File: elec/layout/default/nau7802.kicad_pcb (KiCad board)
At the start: 2 copper layers, 225.7 x 100.8 mm, 0 parts

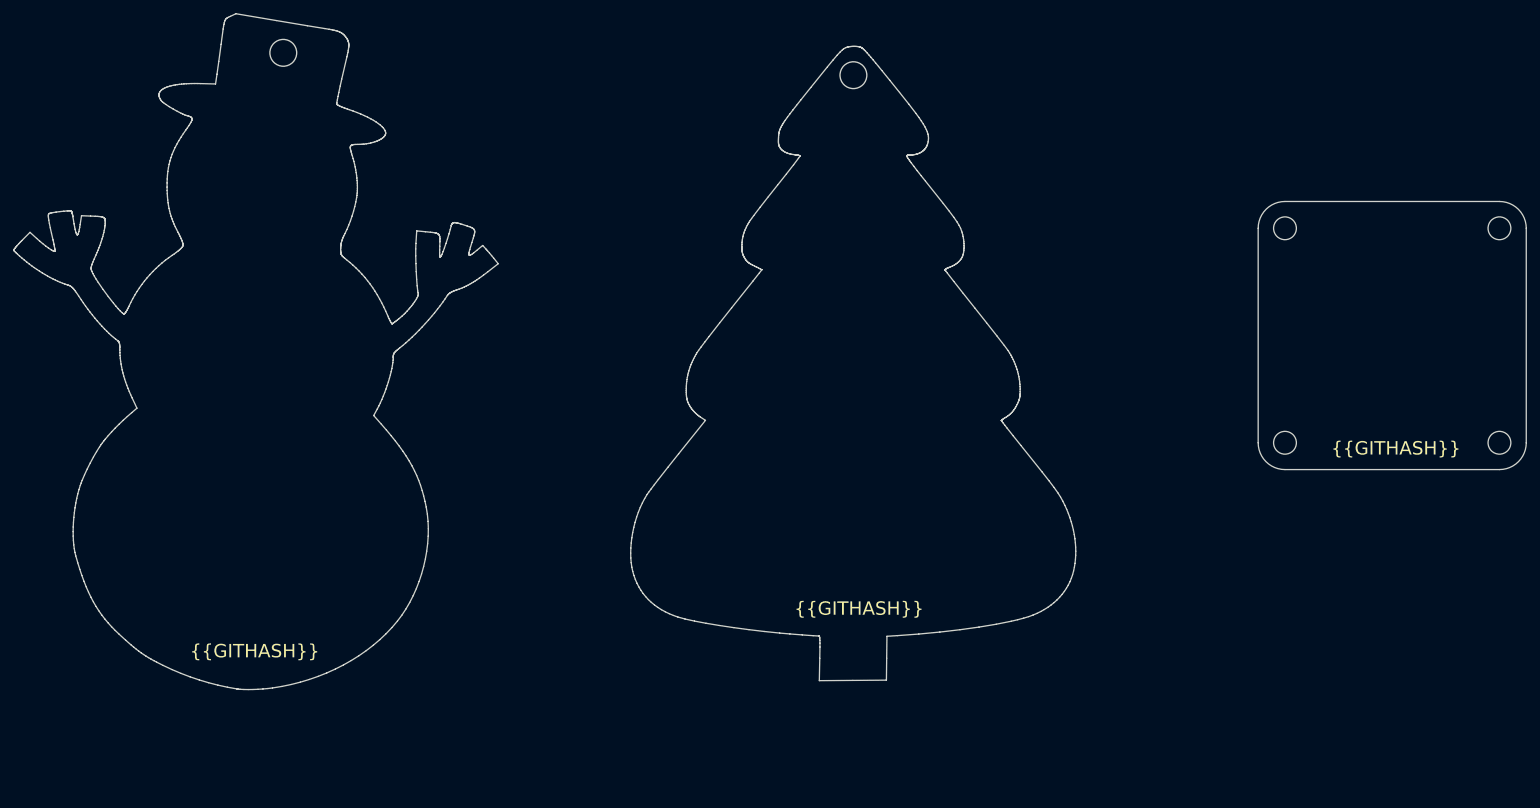
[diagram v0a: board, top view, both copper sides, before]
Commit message: layout
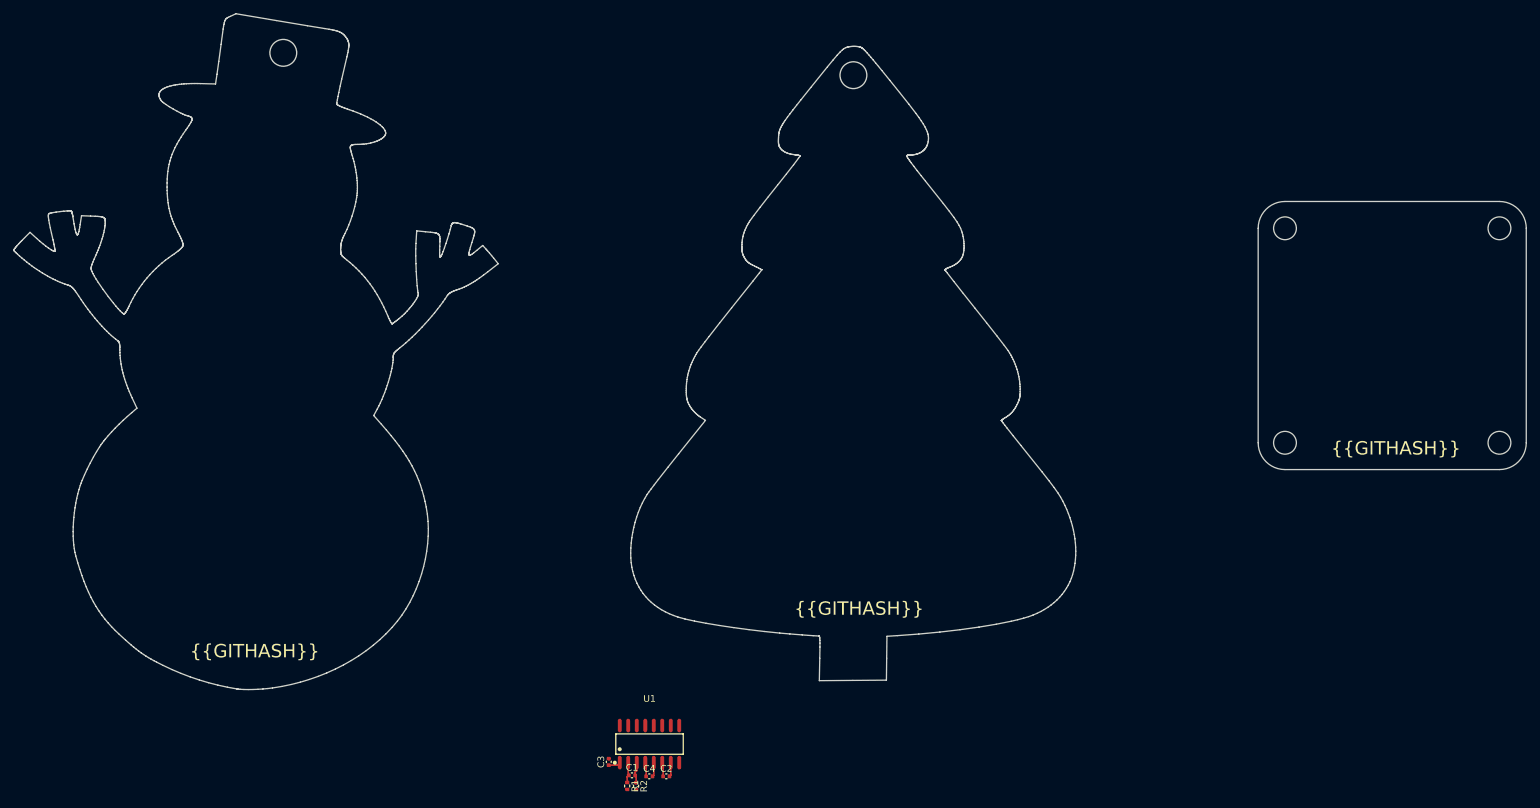
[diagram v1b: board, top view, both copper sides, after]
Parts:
- added C1: Multilayer Ceramic Capacitors MLCC - SMD/SMT 100nF 10V 0402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, lib:C0402, F.Cu at (128.2, 163.4)
- added C2: Multilayer Ceramic Capacitors MLCC - SMD/SMT 100nF 10V 0402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, lib:C0402, F.Cu at (133.3, 163.6)
- added C3: Multilayer Ceramic Capacitors MLCC - SMD/SMT 100nF 10V 0402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, lib:C0402, F.Cu at (124.7, 161.4)
- added C4: Multilayer Ceramic Capacitors MLCC - SMD/SMT 270pF 50V 0402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, lib:C0402, F.Cu at (130.8, 163.6)
- added R1: Chip Resistor - Surface Mount 51Ohms ±5% 1/16W 0402 RoHS, lib:R0402, F.Cu at (127.5, 165.0)
- added R2: Chip Resistor - Surface Mount 51Ohms ±5% 1/16W 0402 RoHS, lib:R0402, F.Cu at (128.8, 165.0)
- added U1: , lib:SOP-16_L9.9-W3.9-P1.27-LS6.0-BL, F.Cu at (130.8, 158.8)
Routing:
- net vin1p: track 0.00 -> 3.15 mm
- net vin1n: track 0.00 -> 3.09 mm
- net vin2p: track 0.00 -> 2.12 mm
- net gnd: track 0.00 -> 2.12 mm
- net vbg: track 0.00 -> 2.10 mm
- net vin2n: track 0.00 -> 2.09 mm
- net refp: track 0.00 -> 1.78 mm
